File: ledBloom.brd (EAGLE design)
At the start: 11.4 x 14.6 mm, 4 parts, among them J1 455-1750-1-ND, J2 455-1750-1-ND, U1 WS2812

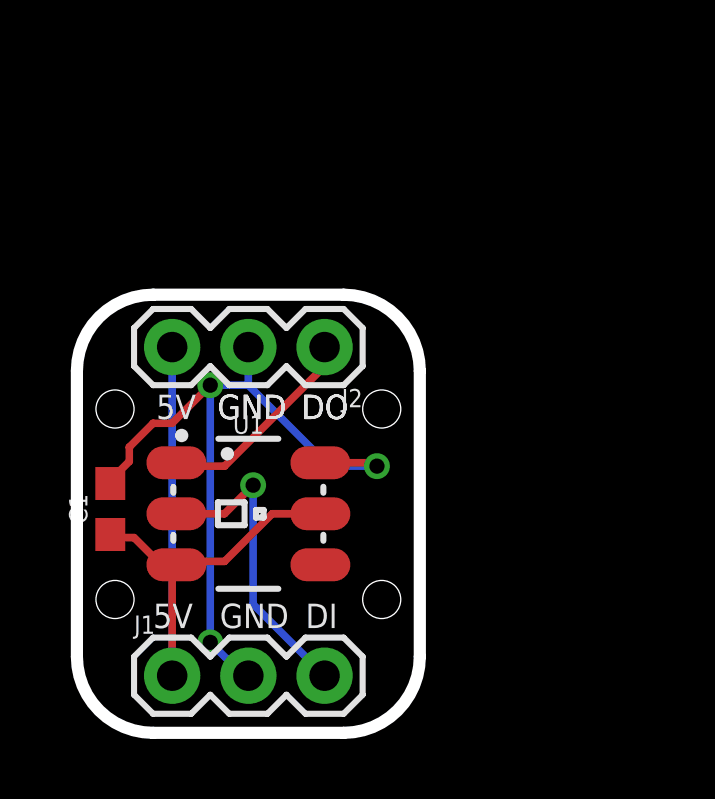
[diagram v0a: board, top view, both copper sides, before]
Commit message: adding production files
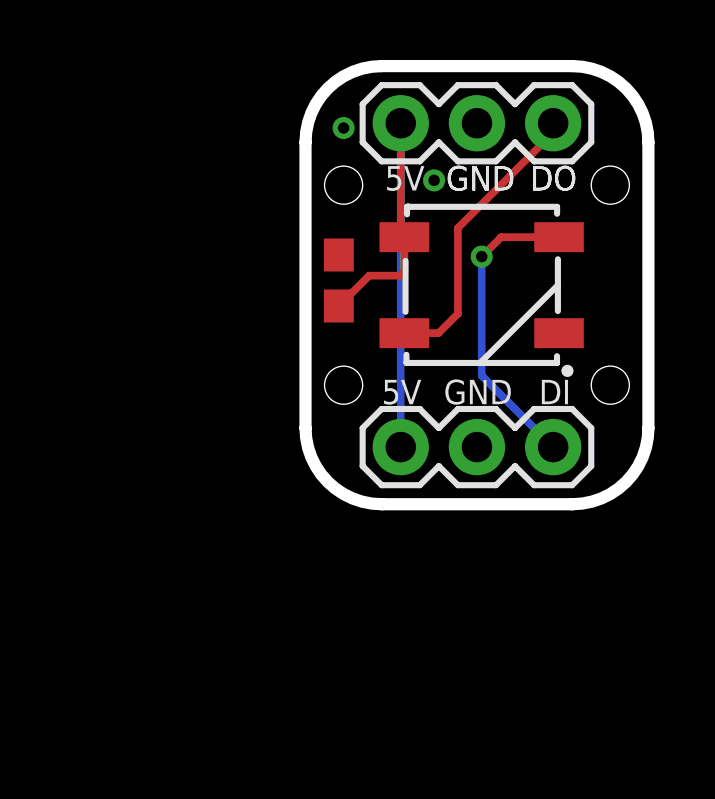
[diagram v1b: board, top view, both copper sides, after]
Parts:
- removed U1: WS2812, SparkFun-LED:LED-TRICOLOR-5050-IC
- added D1: WS2812B, SparkFun-LED:WS2812B
- moved J1 10.8 mm to (5.71, 2.54)
- moved C1 10.8 mm to (3.65, 8.10)
- moved J2 10.7 mm to (10.8, 13.3)
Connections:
- net DI: now also D1.4; no longer U1.2
- net DO: now also D1.2; no longer U1.1
- net GND: now also D1.3; no longer U1.6
- net VCC: now also D1.1; no longer U1.3, U1.5
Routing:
- net GND: track 25.2 -> 0.00 mm, vias 3 -> 2
- net VCC: track 22.8 -> 18.9 mm
- net DO: track 7.00 -> 9.72 mm
